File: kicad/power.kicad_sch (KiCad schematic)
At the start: 44 parts, among them J1 USB_C Connector, J3 START_MODULE, J6 BATT_IN, Q1 Si2371EDS, U1 LMR33630ADDAR, U2 USBLC6-2P6, U4 TLV75733PDBVR

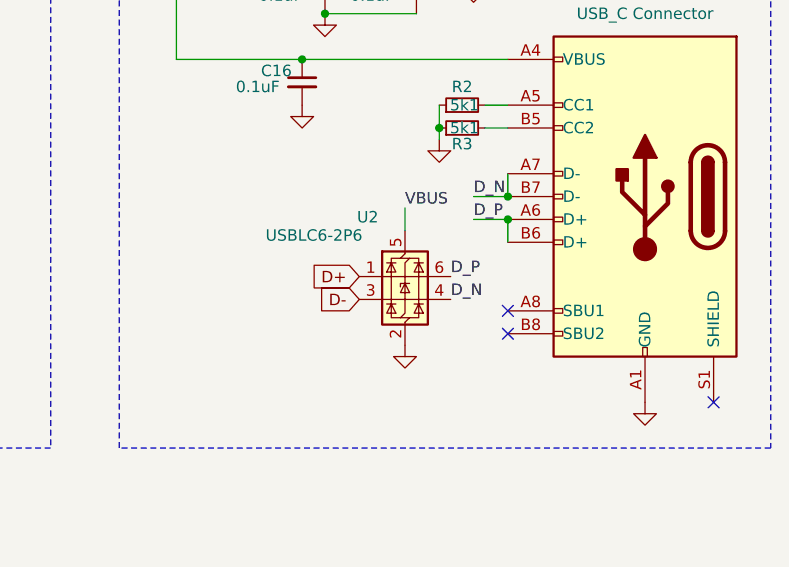
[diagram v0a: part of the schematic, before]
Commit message: 2026 version
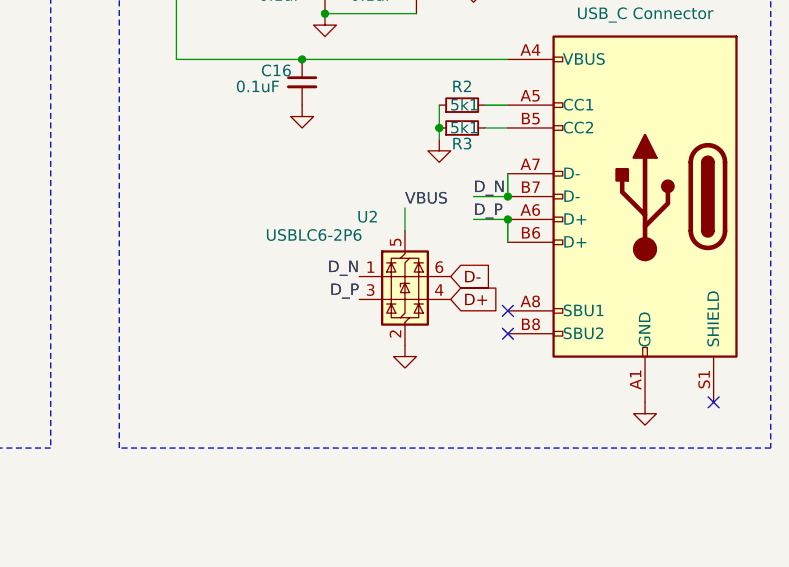
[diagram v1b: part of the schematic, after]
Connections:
- net D+: now also U2.4 (I/O2); no longer U2.1 (I/O1)
- net D-: now also U2.6 (I/O1); no longer U2.3 (I/O2)
- net D_N: now also U2.1 (I/O1); no longer U2.4 (I/O2)
- net D_P: now also U2.3 (I/O2); no longer U2.6 (I/O1)
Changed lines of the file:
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@@
-		)
-	)
-	(label "D_P"
-		(at 240.03 100.33 0)
-		(effects
-			(font
-				(size 1.27 1.27)
-			)
-			(justify left bottom)
 		)
 	)
@@
 		)
 	)
+	(label "D_N"
+		(at 229.87 100.33 180)
+		(effects
+			(font
+				(size 1.27 1.27)
+			)
+			(justify right bottom)
+		)
+	)
 	(label "VBUS"
 		(at 234.95 92.71 0)
@@
 		)
 	)
-	(label "D_N"
-		(at 240.03 102.87 0)
+	(label "D_P"
+		(at 229.87 102.87 180)
 		(effects
 			(font
 				(size 1.27 1.27)
 			)
-			(justify left bottom)
+			(justify right bottom)
 		)
 	)
 	(global_label "D-"
 		(shape input)
-		(at 229.87 102.87 180)
+		(at 240.03 100.33 0)
 		(fields_autoplaced yes)
 		(effects
@@
 				(size 1.27 1.27)
 			)
-			(justify right)
+			(justify left)
 		)
 		(property "Intersheetrefs" "${INTERSHEET_REFS}"
-			(at 224.0424 102.87 0)
+			(at 245.8576 100.33 0)
 			(effects
 				(font
 					(size 1.27 1.27)
 				)
-				(justify right)
+				(justify left)
 				(hide yes)
 			)
@@
 	(global_label "D+"
 		(shape input)
-		(at 229.87 100.33 180)
+		(at 240.03 102.87 0)
 		(fields_autoplaced yes)
 		(effects
@@
 				(size 1.27 1.27)
 			)
-			(justify right)
+			(justify left)
 		)
 		(property "Intersheetrefs" "${INTERSHEET_REFS}"
-			(at 224.0424 100.33 0)
+			(at 245.8576 102.87 0)
 			(effects
 				(font
 					(size 1.27 1.27)
 				)
-				(justify right)
+				(justify left)
 				(hide yes)
 			)
